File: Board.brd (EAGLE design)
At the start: 47 x 35 mm, 57 parts, among them IC1 CP210X_USB_UART, T1 BC846, T2 BC846

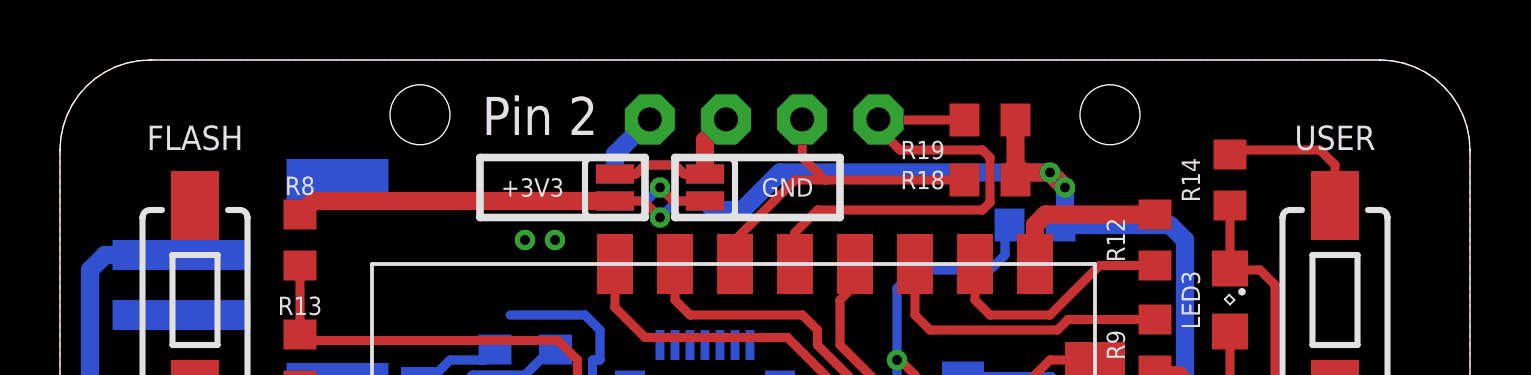
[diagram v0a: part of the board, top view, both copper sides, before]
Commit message: cleanup schematic
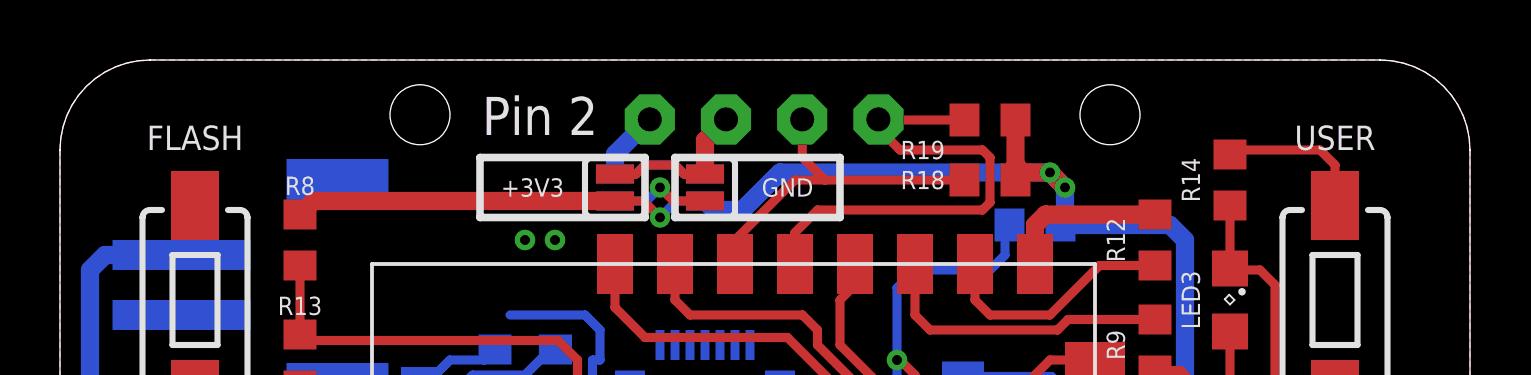
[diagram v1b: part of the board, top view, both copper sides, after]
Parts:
- R1, R2: value (none) -> 470
- R16: value 220k -> 50k
- R17: value 100k -> 220k
